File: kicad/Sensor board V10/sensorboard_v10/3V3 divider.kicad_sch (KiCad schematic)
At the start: 4 parts, among them J16 Conn_01x03

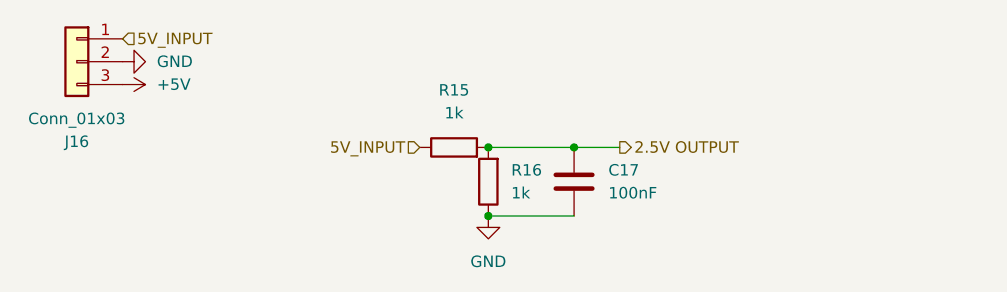
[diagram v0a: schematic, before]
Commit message: Sensor Board v10
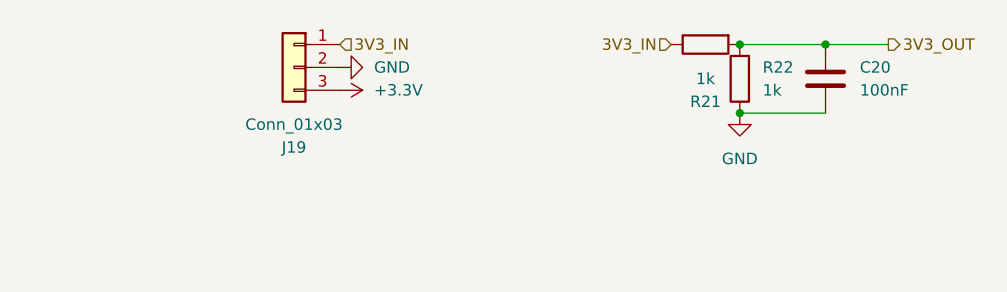
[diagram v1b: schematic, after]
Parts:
- removed C17: 100nF, RMC_Capacitor:C_0805_2012Metric_Pad1.18x1.45mm_HandSolder_L, symbol Device:C
- removed J16: Conn_01x03, Connector_JST:JST_XH_B3B-XH-A_1x03_P2.50mm_Vertical, symbol Connector_Generic:Conn_01x03
- removed R15, R16: 1k, RMC_Resistor:R_0805_2012Metric_Pad1.20x1.40mm_HandSolder_L, symbol Device:R
- added C20: 100nF, RMC_Capacitor:C_0805_2012Metric_Pad1.18x1.45mm_HandSolder_L, symbol Device:C
- added J19: Conn_01x03, Connector_JST:JST_XH_B3B-XH-A_1x03_P2.50mm_Vertical, symbol Connector_Generic:Conn_01x03
- added R21, R22: 1k, RMC_Resistor:R_0805_2012Metric_Pad1.20x1.40mm_HandSolder_L, symbol Device:R
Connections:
- net GND: now also C20.1, J19.2 (Pin_2), R22.1
- new net +3.3V: J19.3 (Pin_3)
- new net 3V3_IN: J19.1 (Pin_1), R21.1
- new net 3V3_OUT: C20.2, R21.2, R22.2
